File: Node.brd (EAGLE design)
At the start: 27.9 x 27.9 mm, 60 parts, among them J1 DF12A3.0-14DS, Q1 16MHz, U1 ATMEGA32U4QFN, U2 NRF24L01NOPAD, U3 LTC3553, U4 L3GD20, U6 LSM303DLHC, U7 BD2425NNRF0404, U9 RCLAMP0502A, X1 USB-FCI

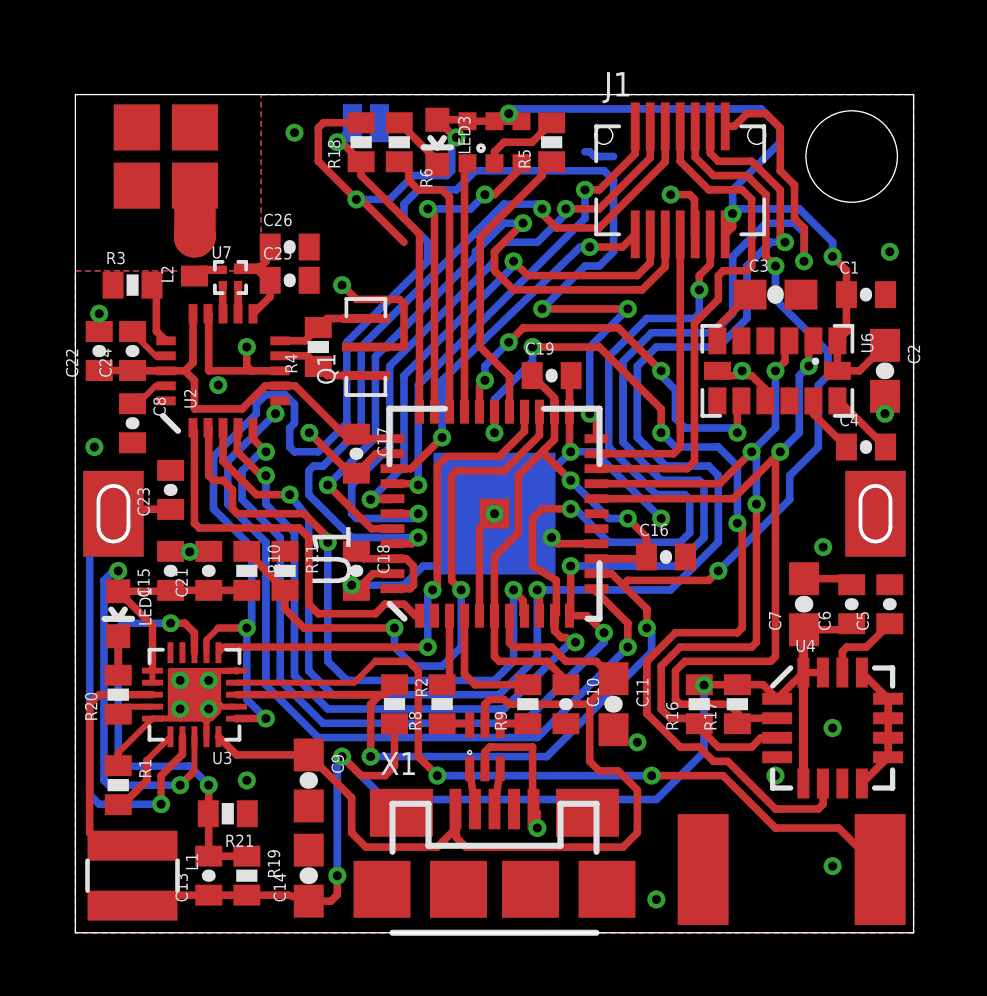
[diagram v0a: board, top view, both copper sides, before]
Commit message: 7 more to go
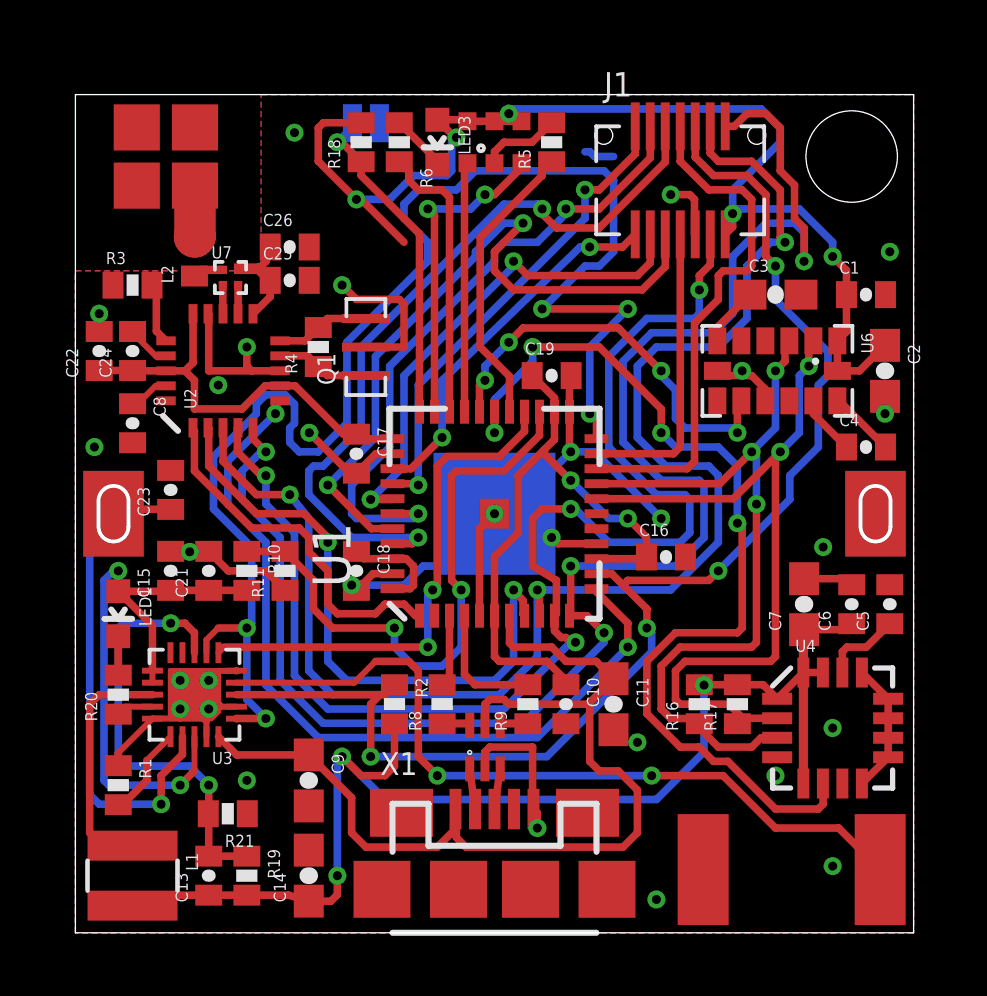
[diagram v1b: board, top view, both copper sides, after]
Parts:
- turned R11 to 90 degrees
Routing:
- net GND: track 64.8 -> 67.9 mm
- net CE: track 13.5 -> 12.1 mm
- net SS: track 21.0 -> 20.5 mm
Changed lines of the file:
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@@
 <element name="R20" library="SparkFun" package="0402-RES" value="1k" x="1.42875" y="7.9375" rot="R90"/>
 <element name="R10" library="SparkFun" package="0402-RES" value="100k" x="5.715" y="12.065" rot="R270"/>
-<element name="R11" library="SparkFun" package="0402-RES" value="100k" x="6.985" y="12.065" rot="R270"/>
+<element name="R11" library="SparkFun" package="0402-RES" value="100k" x="6.985" y="12.065" rot="R90"/>
 <element name="R1" library="SparkFun" package="0402-RES" value="7.5k" x="1.42875" y="4.92125" rot="R270"/>
 <element name="C13" library="SparkFun" package="0402-CAP" value="10pF" x="4.445" y="1.905" rot="R90"/>
@@
 <wire x1="17.145" y1="26.035" x2="17.30375" y2="25.87625" width="0.254" layer="16"/>
 <wire x1="17.30375" y1="25.87625" x2="17.93875" y2="25.87625" width="0.254" layer="16"/>
+<wire x1="6.985" y1="11.415" x2="6.985" y2="11.43" width="0.254" layer="1"/>
+<wire x1="6.985" y1="11.43" x2="6.35" y2="12.065" width="0.254" layer="1"/>
+<wire x1="6.35" y1="12.065" x2="5.095" y2="12.065" width="0.254" layer="1"/>
+<wire x1="5.095" y1="12.065" x2="4.445" y2="12.715" width="0.254" layer="1"/>
 <wire x1="27.0025" y1="21.2725" x2="24.18625" y2="21.2725" width="0" layer="19" extent="1-1"/>
-<wire x1="6.985" y1="12.715" x2="9.2075" y2="11.57375" width="0" layer="19" extent="1-1"/>
 </signal>
 <signal name="+3V3">
@@
 <contactref element="R11" pad="2"/>
 <contactref element="U1" pad="25"/>
-<wire x1="6.985" y1="11.415" x2="5.715" y2="12.715" width="0.254" layer="1"/>
+<wire x1="6.985" y1="12.715" x2="5.715" y2="12.715" width="0.254" layer="1"/>
 <wire x1="15.47" y1="17.37" x2="15.47" y2="16.58125" width="0.254" layer="1"/>
 <wire x1="15.47" y1="16.58125" x2="14.2875" y2="15.39875" width="0.254" layer="1"/>
@@
 <wire x1="10.63625" y1="9.525" x2="10.63625" y2="10.16" width="0.254" layer="16"/>
 <via x="10.63625" y="10.16" extent="1-16" drill="0.3"/>
-<wire x1="10.63625" y1="10.16" x2="7.62" y2="10.16" width="0.254" layer="1"/>
-<wire x1="7.62" y1="10.16" x2="6.985" y2="10.795" width="0.254" layer="1"/>
-<wire x1="6.985" y1="10.795" x2="6.985" y2="11.415" width="0.254" layer="1"/>
+<wire x1="10.63625" y1="10.16" x2="8.5725" y2="10.16" width="0.254" layer="1"/>
+<wire x1="8.5725" y1="10.16" x2="7.9375" y2="10.795" width="0.254" layer="1"/>
+<wire x1="7.9375" y1="10.795" x2="7.9375" y2="11.7475" width="0.254" layer="1"/>
+<wire x1="7.9375" y1="11.7475" x2="6.985" y2="12.715" width="0.254" layer="1"/>
 </signal>
 <signal name="N$29">
@@
 <wire x1="9.04875" y1="19.685" x2="9.04875" y2="16.98625" width="0.254" layer="16"/>
 <wire x1="9.04875" y1="16.98625" x2="8.09625" y2="16.03375" width="0.254" layer="16"/>
-<wire x1="8.09625" y1="16.03375" x2="7.3025" y2="16.03375" width="0.254" layer="16"/>
-<wire x1="7.3025" y1="16.03375" x2="7.14375" y2="16.1925" width="0.254" layer="16"/>
-<wire x1="7.14375" y1="16.1925" x2="7.14375" y2="16.8275" width="0.254" layer="16"/>
+<wire x1="8.09625" y1="16.03375" x2="7.46125" y2="16.03375" width="0.254" layer="16"/>
+<wire x1="7.46125" y1="16.03375" x2="7.14375" y2="16.35125" width="0.254" layer="16"/>
+<wire x1="7.14375" y1="16.35125" x2="7.14375" y2="16.8275" width="0.254" layer="16"/>
 <wire x1="7.14375" y1="16.8275" x2="7.3025" y2="16.98625" width="0.254" layer="16"/>
 <wire x1="7.3025" y1="16.98625" x2="7.3025" y2="17.62125" width="0.254" layer="16"/>
@@
 <contactref element="U2" pad="2"/>
 <wire x1="4.42125" y1="16.8325" x2="4.445" y2="16.80875" width="0.254" layer="1"/>
-<wire x1="4.445" y1="16.80875" x2="4.445" y2="15.24" width="0.254" layer="1"/>
-<wire x1="4.445" y1="15.24" x2="4.60375" y2="15.08125" width="0.254" layer="1"/>
-<wire x1="4.60375" y1="15.08125" x2="4.92125" y2="15.08125" width="0.254" layer="1"/>
-<wire x1="4.92125" y1="15.08125" x2="5.23875" y2="14.76375" width="0.254" layer="1"/>
-<wire x1="5.23875" y1="14.76375" x2="5.23875" y2="14.12875" width="0.254" layer="1"/>
-<wire x1="5.23875" y1="14.12875" x2="5.3975" y2="13.97" width="0.254" layer="1"/>
-<wire x1="5.3975" y1="13.97" x2="7.62" y2="13.97" width="0.254" layer="1"/>
+<wire x1="4.445" y1="16.80875" x2="4.445" y2="15.5575" width="0.254" layer="1"/>
+<wire x1="4.445" y1="15.5575" x2="6.0325" y2="13.97" width="0.254" layer="1"/>
+<wire x1="6.0325" y1="13.97" x2="7.62" y2="13.97" width="0.254" layer="1"/>
 <wire x1="7.62" y1="13.97" x2="8.41375" y2="13.17625" width="0.254" layer="1"/>
 <wire x1="8.41375" y1="13.17625" x2="8.41375" y2="13.0175" width="0.254" layer="1"/>
@@
 <contactref element="U2" pad="1"/>
 <wire x1="3.92125" y1="16.8325" x2="3.96875" y2="16.72125" width="0.254" layer="1"/>
-<wire x1="3.96875" y1="16.72125" x2="3.96875" y2="13.6525" width="0.254" layer="1"/>
-<wire x1="3.96875" y1="13.6525" x2="4.1275" y2="13.49375" width="0.254" layer="1"/>
-<wire x1="4.1275" y1="13.49375" x2="7.46125" y2="13.49375" width="0.254" layer="1"/>
+<wire x1="3.96875" y1="16.72125" x2="3.96875" y2="15.39875" width="0.254" layer="1"/>
+<wire x1="3.96875" y1="15.39875" x2="5.87375" y2="13.49375" width="0.254" layer="1"/>
+<wire x1="5.87375" y1="13.49375" x2="7.46125" y2="13.49375" width="0.254" layer="1"/>
 <wire x1="7.46125" y1="13.49375" x2="7.77875" y2="13.17625" width="0.254" layer="1"/>
-<wire x1="7.77875" y1="13.17625" x2="7.77875" y2="10.95375" width="0.254" layer="1"/>
-<wire x1="7.77875" y1="10.95375" x2="8.09625" y2="10.63625" width="0.254" layer="1"/>
-<wire x1="8.09625" y1="10.63625" x2="10.00125" y2="10.63625" width="0.254" layer="1"/>
+<wire x1="7.77875" y1="13.17625" x2="7.77875" y2="12.7" width="0.254" layer="1"/>
+<wire x1="7.77875" y1="12.7" x2="8.41375" y2="12.065" width="0.254" layer="1"/>
+<wire x1="8.41375" y1="12.065" x2="8.41375" y2="10.95375" width="0.254" layer="1"/>
+<wire x1="8.41375" y1="10.95375" x2="8.73125" y2="10.63625" width="0.254" layer="1"/>
+<wire x1="8.73125" y1="10.63625" x2="10.00125" y2="10.63625" width="0.254" layer="1"/>
 <wire x1="10.00125" y1="10.63625" x2="10.31875" y2="10.95375" width="0.254" layer="1"/>
 <wire x1="10.31875" y1="10.95375" x2="10.95375" y2="10.95375" width="0.254" layer="1"/>
